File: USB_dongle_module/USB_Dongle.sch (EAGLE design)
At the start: 18 parts, among them IC1 FT232RQ, IC2 LM50, X1 USB-A

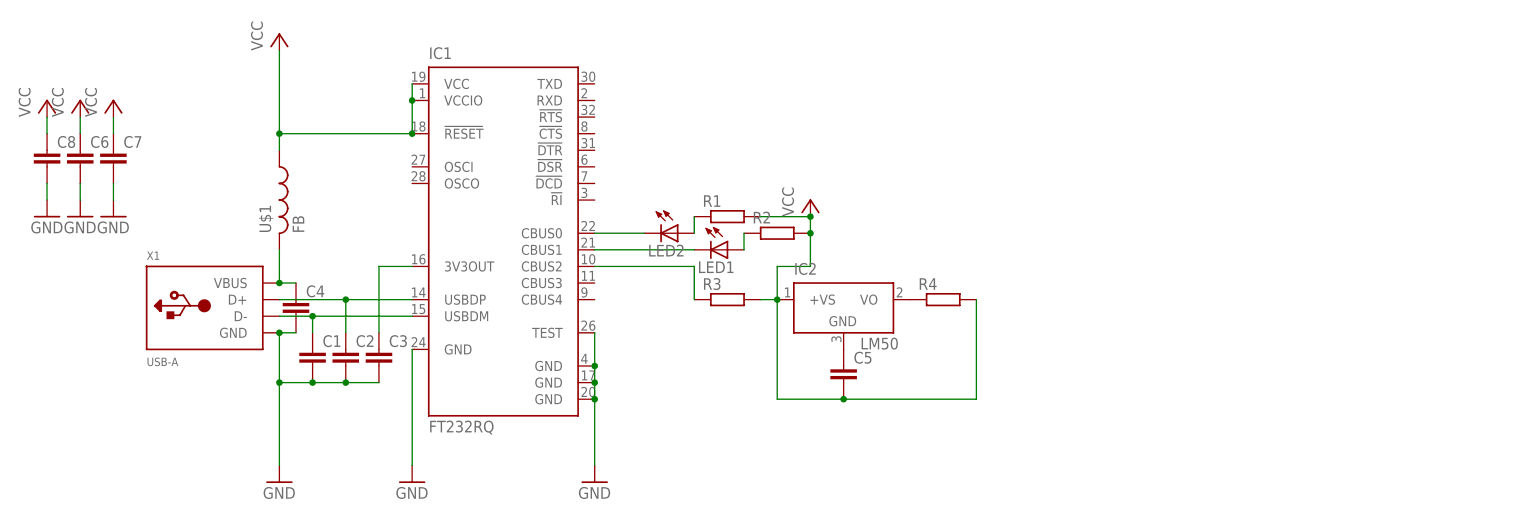
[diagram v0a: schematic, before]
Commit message: Skeem
Skeem valmis, vaja lisada nimetused ja väärtused
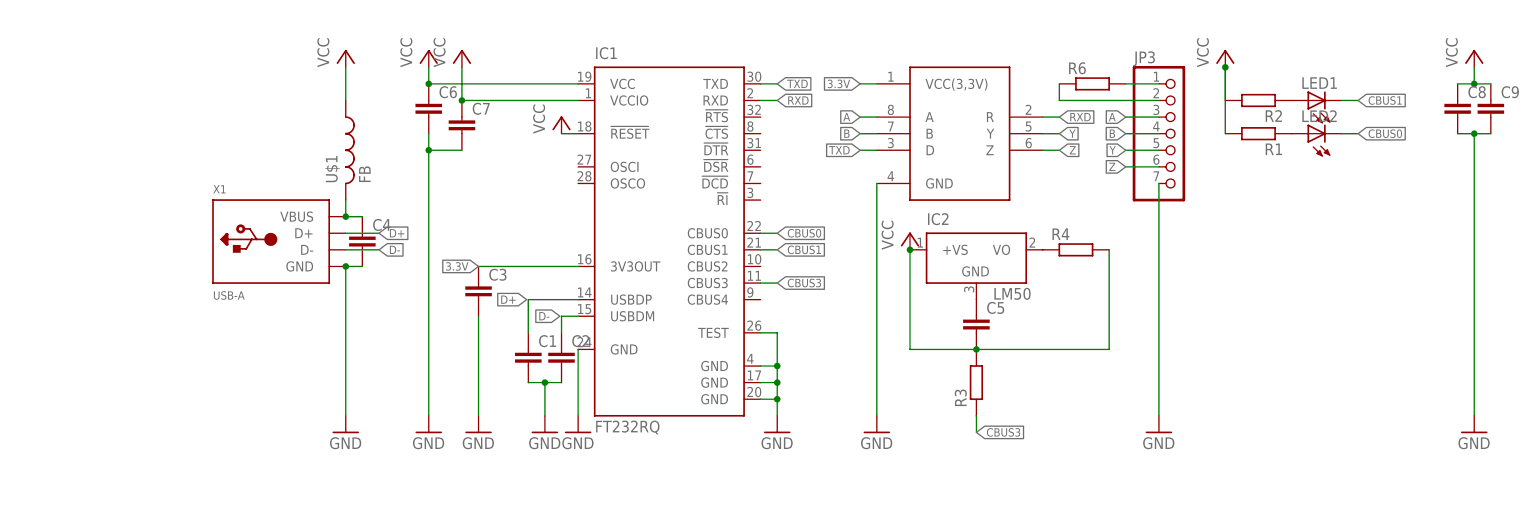
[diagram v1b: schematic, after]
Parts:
- added C9: (no value), eagle-ltspice:CC0603
- added JP3: (no value), pinhead:PINHD-1X7
- added R6: (no value), resistor:R-EU_R0603
- added U$2: SN65HVD77D, Kommunikatsioon:SN65HVD77D
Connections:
- net N$5 renamed CBUS0
- net N$6 renamed CBUS1
- removed net N$10: IC1.CBUS2, R3.1
- removed net N$4: C3.1, IC1.3V3OUT
- new net 3.3V: C3.1, IC1.3V3OUT, U$2.VCC(3,3V)
- new net A: JP3.3, U$2.A
- new net B: JP3.4, U$2.B
- new net CBUS3: IC1.CBUS3, R3.1
- new net D+: C1.1, IC1.USBDP, X1.D+
- new net D-: C2.1, IC1.USBDM, X1.D-
- new net N$9: JP3.1, R6.2
- new net RXD: IC1.RXD, U$2.R
- new net TXD: IC1.TXD, U$2.D
- new net Y: JP3.5, U$2.Y
- new net Z: JP3.6, U$2.Z
- net GND: now also C9.2, JP3.7, U$2.GND
- net N$2: now also JP3.2, R6.1; no longer C1.1, IC1.USBDM, X1.D-
- net N$3: now also IC1.!RESET; no longer C2.1, IC1.USBDP, X1.D+
- net VCC: now also C9.1; no longer IC1.!RESET
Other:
- moved on the sheet: C1, C2, C3, C4, C5, C6, C7, C8, IC1, IC2, LED1, LED2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
